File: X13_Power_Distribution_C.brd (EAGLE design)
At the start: 152.4 x 73.7 mm, 34 parts, among them Q1 IRF1018EPBF, Q2 310mA/60V/1.6Ω, Q3 IRF1018EPBF, Q4 IRF1018EPBF

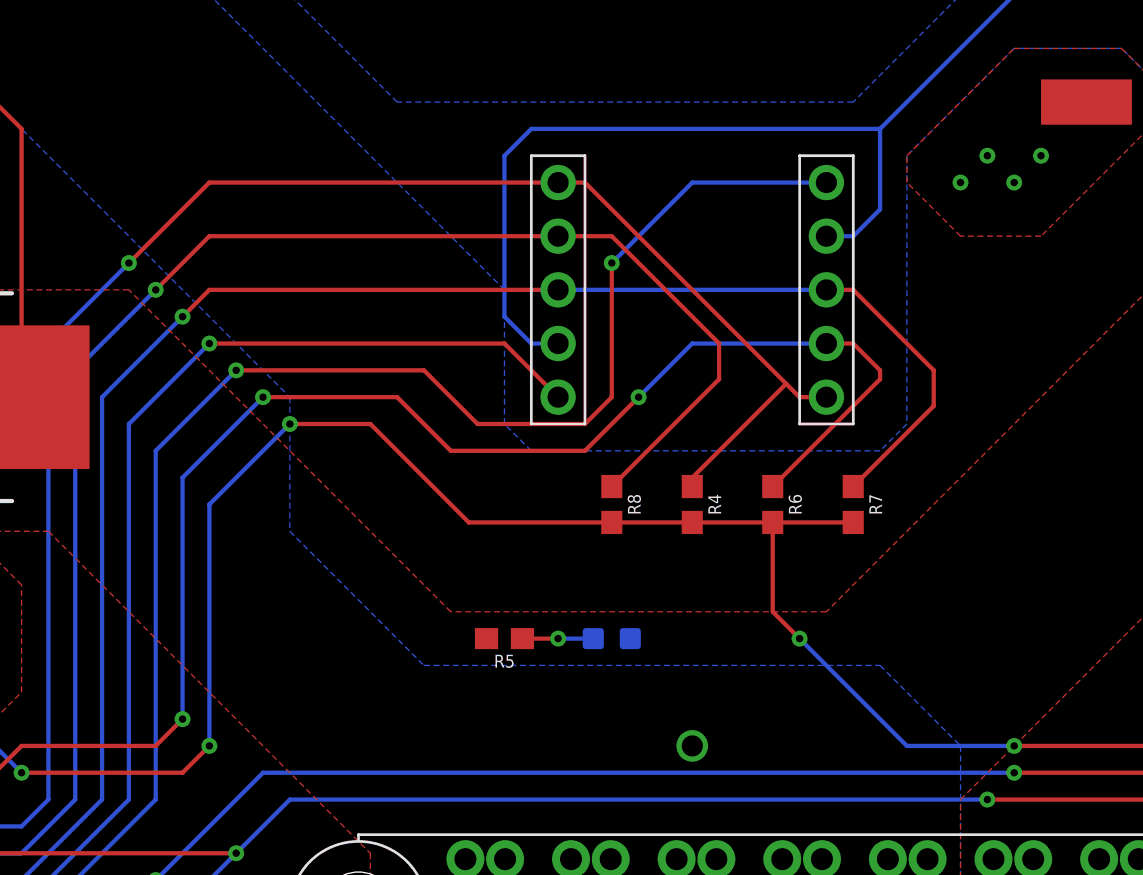
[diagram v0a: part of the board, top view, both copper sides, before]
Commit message: Version C! Uses connector C!
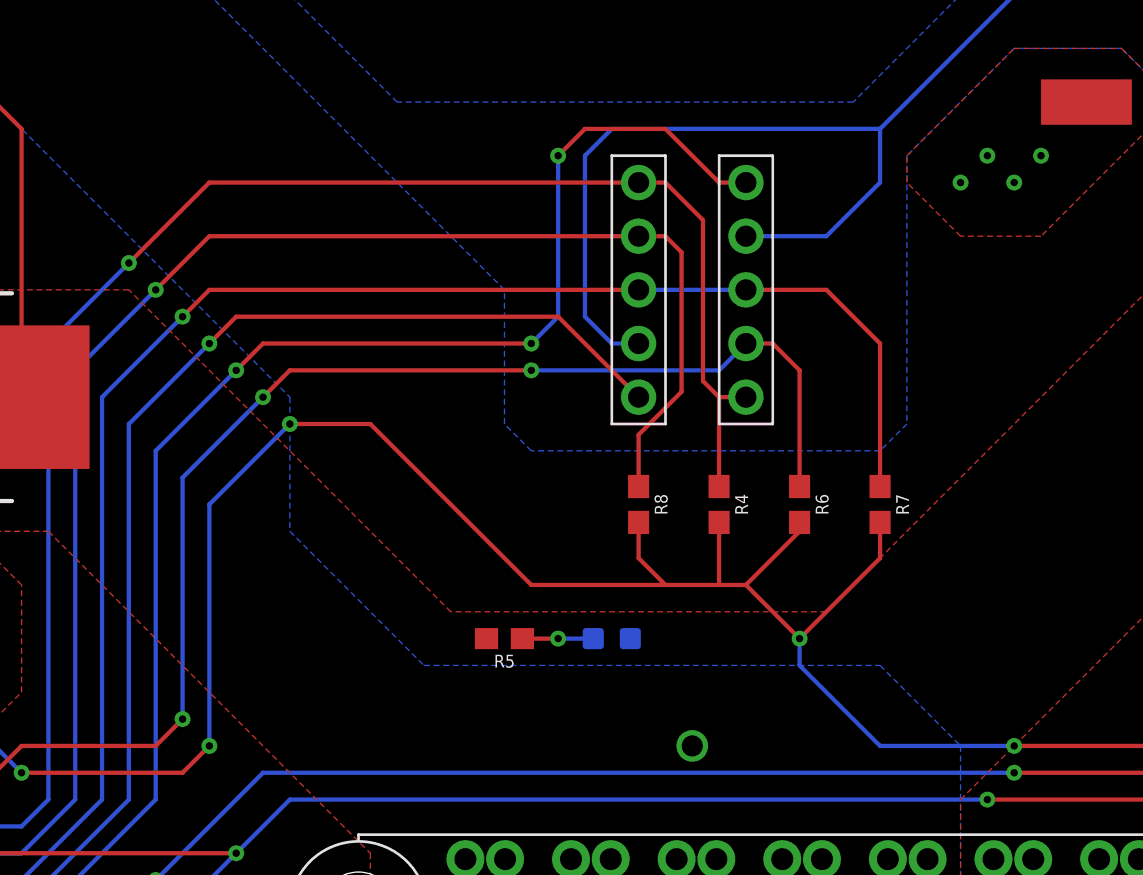
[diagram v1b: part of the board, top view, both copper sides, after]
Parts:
- removed BRICK1, BRICK2: DIST2BRICK_B, Brick_Dist_Connector:DIST2BRICK_B
- added BRICK_A, BRICK_B: DIST2BRICK_C, Brick_Dist_Connector:DIST2BRICK_C
- moved R7 1.27 mm to (85.1, 24.1)
- moved R4 1.27 mm to (77.5, 24.1)
- moved R6 1.27 mm to (81.3, 24.1)
- moved R8 1.27 mm to (73.7, 24.1)
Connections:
- net +12V_A: now also BRICK_A.2@1, BRICK_A.2@10, BRICK_A.2@11, BRICK_A.2@12, BRICK_A.2@13, BRICK_A.2@14, BRICK_A.2@15, BRICK_A.2@16, BRICK_A.2@2, BRICK_A.2@3, BRICK_A.2@4, BRICK_A.2@5, BRICK_A.2@6, BRICK_A.2@7, BRICK_A.2@8, BRICK_A.2@9; no longer BRICK1.2@1, BRICK1.2@10, BRICK1.2@11, BRICK1.2@12, BRICK1.2@13, BRICK1.2@14, BRICK1.2@15, BRICK1.2@16, BRICK1.2@2, BRICK1.2@3, BRICK1.2@4, BRICK1.2@5, BRICK1.2@6, BRICK1.2@7, BRICK1.2@8, BRICK1.2@9
- net +12V_B: now also BRICK_B.2@1, BRICK_B.2@10, BRICK_B.2@11, BRICK_B.2@12, BRICK_B.2@13, BRICK_B.2@14, BRICK_B.2@15, BRICK_B.2@16, BRICK_B.2@2, BRICK_B.2@3, BRICK_B.2@4, BRICK_B.2@5, BRICK_B.2@6, BRICK_B.2@7, BRICK_B.2@8, BRICK_B.2@9; no longer BRICK2.2@1, BRICK2.2@10, BRICK2.2@11, BRICK2.2@12, BRICK2.2@13, BRICK2.2@14, BRICK2.2@15, BRICK2.2@16, BRICK2.2@2, BRICK2.2@3, BRICK2.2@4, BRICK2.2@5, BRICK2.2@6, BRICK2.2@7, BRICK2.2@8, BRICK2.2@9
- net +48V: now also BRICK_A.1@1, BRICK_A.1@10, BRICK_A.1@2, BRICK_A.1@3, BRICK_A.1@4, BRICK_A.1@5, BRICK_A.1@6, BRICK_A.1@7, BRICK_A.1@8, BRICK_A.1@9, BRICK_B.1@1, BRICK_B.1@10, BRICK_B.1@2, BRICK_B.1@3, BRICK_B.1@4, BRICK_B.1@5, BRICK_B.1@6, BRICK_B.1@7, BRICK_B.1@8, BRICK_B.1@9; no longer BRICK1.1@1, BRICK1.1@10, BRICK1.1@2, BRICK1.1@3, BRICK1.1@4, BRICK1.1@5, BRICK1.1@6, BRICK1.1@7, BRICK1.1@8, BRICK1.1@9, BRICK2.1@1, BRICK2.1@10, BRICK2.1@2, BRICK2.1@3, BRICK2.1@4, BRICK2.1@5, BRICK2.1@6, BRICK2.1@7, BRICK2.1@8, BRICK2.1@9
- net 12V_GND: now also BRICK_A.4@1, BRICK_A.4@10, BRICK_A.4@11, BRICK_A.4@12, BRICK_A.4@13, BRICK_A.4@14, BRICK_A.4@15, BRICK_A.4@16, BRICK_A.4@2, BRICK_A.4@3, BRICK_A.4@4, BRICK_A.4@5, BRICK_A.4@6, BRICK_A.4@7, BRICK_A.4@8, BRICK_A.4@9, BRICK_B.4@1, BRICK_B.4@10, BRICK_B.4@11, BRICK_B.4@12, BRICK_B.4@13, BRICK_B.4@14, BRICK_B.4@15, BRICK_B.4@16, BRICK_B.4@2, BRICK_B.4@3, BRICK_B.4@4, BRICK_B.4@5, BRICK_B.4@6, BRICK_B.4@7, BRICK_B.4@8, BRICK_B.4@9; no longer BRICK1.4@1, BRICK1.4@10, BRICK1.4@11, BRICK1.4@12, BRICK1.4@13, BRICK1.4@14, BRICK1.4@15, BRICK1.4@16, BRICK1.4@2, BRICK1.4@3, BRICK1.4@4, BRICK1.4@5, BRICK1.4@6, BRICK1.4@7, BRICK1.4@8, BRICK1.4@9, BRICK2.4@1, BRICK2.4@10, BRICK2.4@11, BRICK2.4@12, BRICK2.4@13, BRICK2.4@14, BRICK2.4@15, BRICK2.4@16, BRICK2.4@2, BRICK2.4@3, BRICK2.4@4, BRICK2.4@5, BRICK2.4@6, BRICK2.4@7, BRICK2.4@8, BRICK2.4@9
- net 48V_GND: now also BRICK_A.3@1, BRICK_A.3@10, BRICK_A.3@2, BRICK_A.3@3, BRICK_A.3@4, BRICK_A.3@5, BRICK_A.3@6, BRICK_A.3@7, BRICK_A.3@8, BRICK_A.3@9, BRICK_B.3@1, BRICK_B.3@10, BRICK_B.3@2, BRICK_B.3@3, BRICK_B.3@4, BRICK_B.3@5, BRICK_B.3@6, BRICK_B.3@7, BRICK_B.3@8, BRICK_B.3@9; no longer BRICK1.3@1, BRICK1.3@10, BRICK1.3@2, BRICK1.3@3, BRICK1.3@4, BRICK1.3@5, BRICK1.3@6, BRICK1.3@7, BRICK1.3@8, BRICK1.3@9, BRICK2.3@1, BRICK2.3@10, BRICK2.3@2, BRICK2.3@3, BRICK2.3@4, BRICK2.3@5, BRICK2.3@6, BRICK2.3@7, BRICK2.3@8, BRICK2.3@9
- net ALERT_1: now also BRICK_A.D; no longer BRICK1.D
- net ALERT_2: now also BRICK_B.D; no longer BRICK2.D
- net C2_1: now also BRICK_A.A; no longer BRICK1.A
- net C2_2: now also BRICK_B.A; no longer BRICK2.A
- net CLK: now also BRICK_A.C, BRICK_B.C; no longer BRICK1.C, BRICK2.C
- net DATA: now also BRICK_A.E, BRICK_B.E; no longer BRICK1.E, BRICK2.E
- net ON/OFF: now also BRICK_A.B, BRICK_B.B; no longer BRICK1.B, BRICK2.B
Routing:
- net +3.3V: track 142.4 -> 154.4 mm
- net ALERT_2: track 78.5 -> 70.5 mm
- net C2_1: track 66.0 -> 70.9 mm
- net CLK: track 89.6 -> 86.2 mm
- net C2_2: track 89.5 -> 86.4 mm, vias 2 -> 3
- net DATA: track 80.6 -> 79.2 mm
- net ON/OFF: track 79.4 -> 78.6 mm
- net ALERT_1: track 77.4 -> 76.9 mm
